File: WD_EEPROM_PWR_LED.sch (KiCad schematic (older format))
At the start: 40 parts, among them IC19 TPS3430WDRCR, IC20 M24C64-DRDW8TP_K, J16 Conn_01x03, Q22 DMN26D0UFB4-7, Q23 DMN26D0UFB4-7, Q24 DMN26D0UFB4-7, Q25 DMN26D0UFB4-7, Q26 DMN26D0UFB4-7, Q27 DMN26D0UFB4-7, Q28 DMN26D0UFB4-7, Q29 DMN26D0UFB4-7

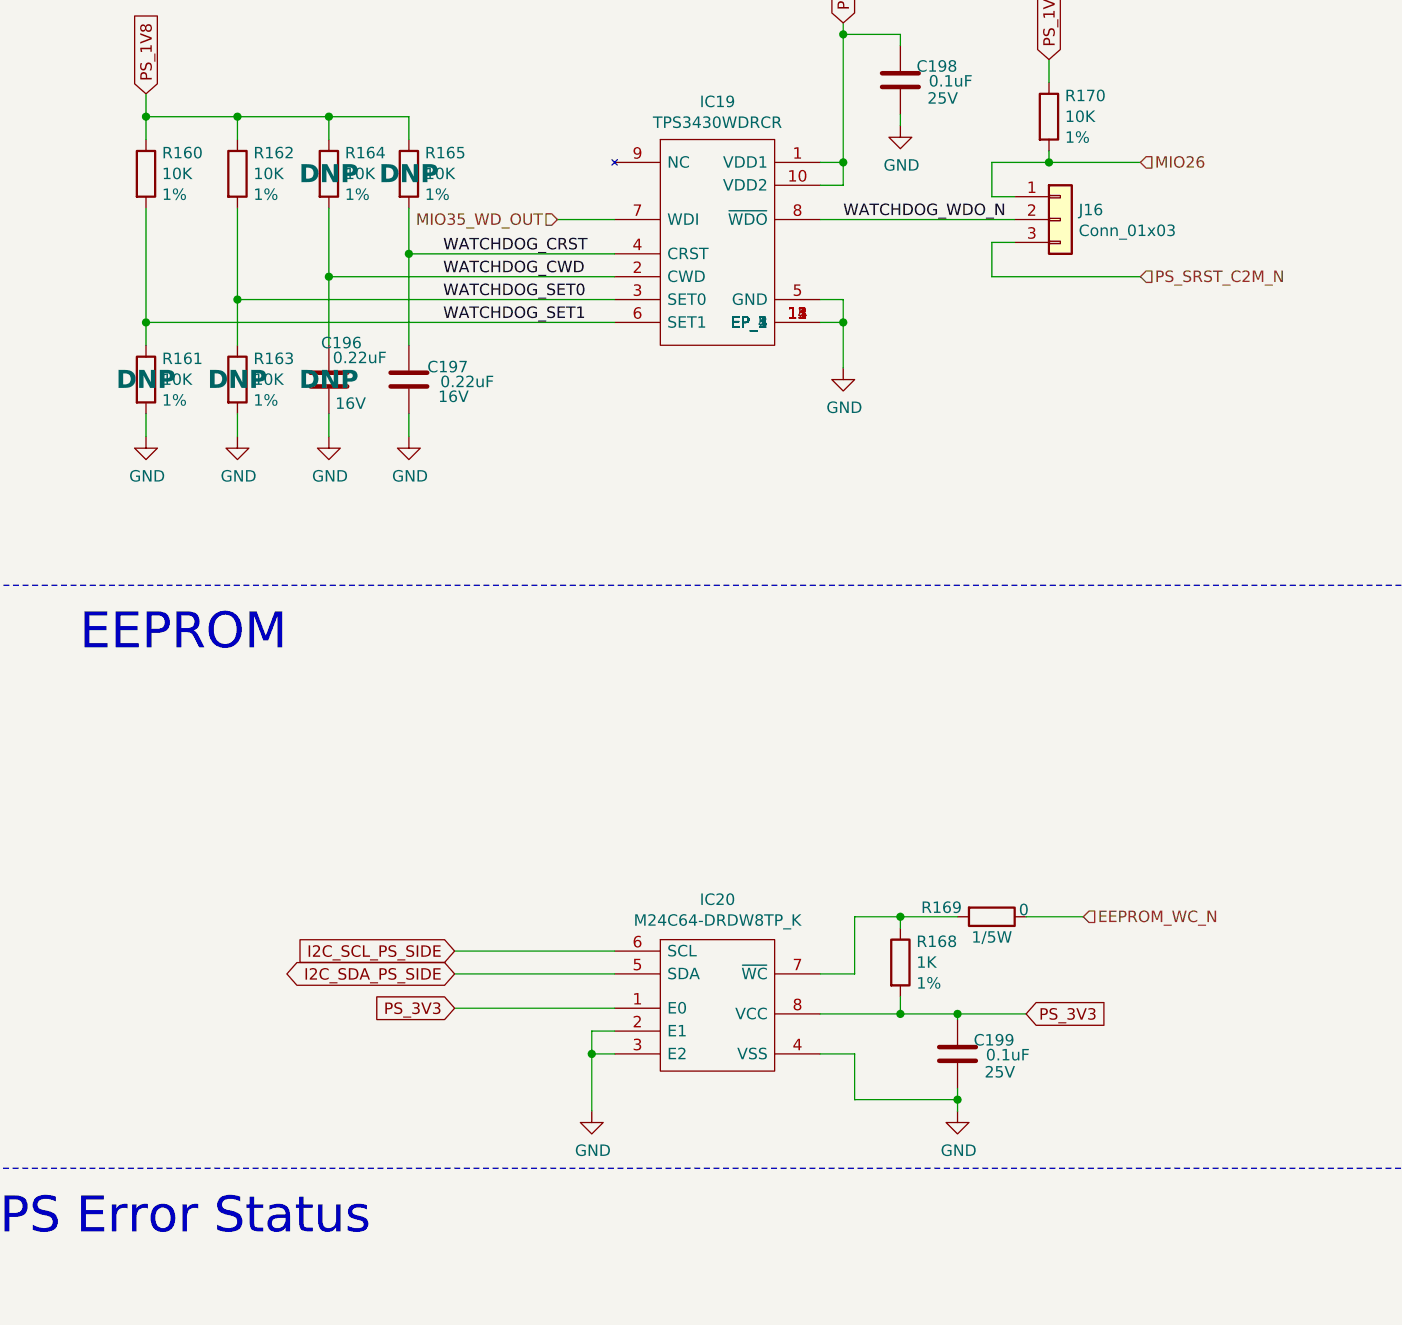
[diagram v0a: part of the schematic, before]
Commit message: Pre-Production Push
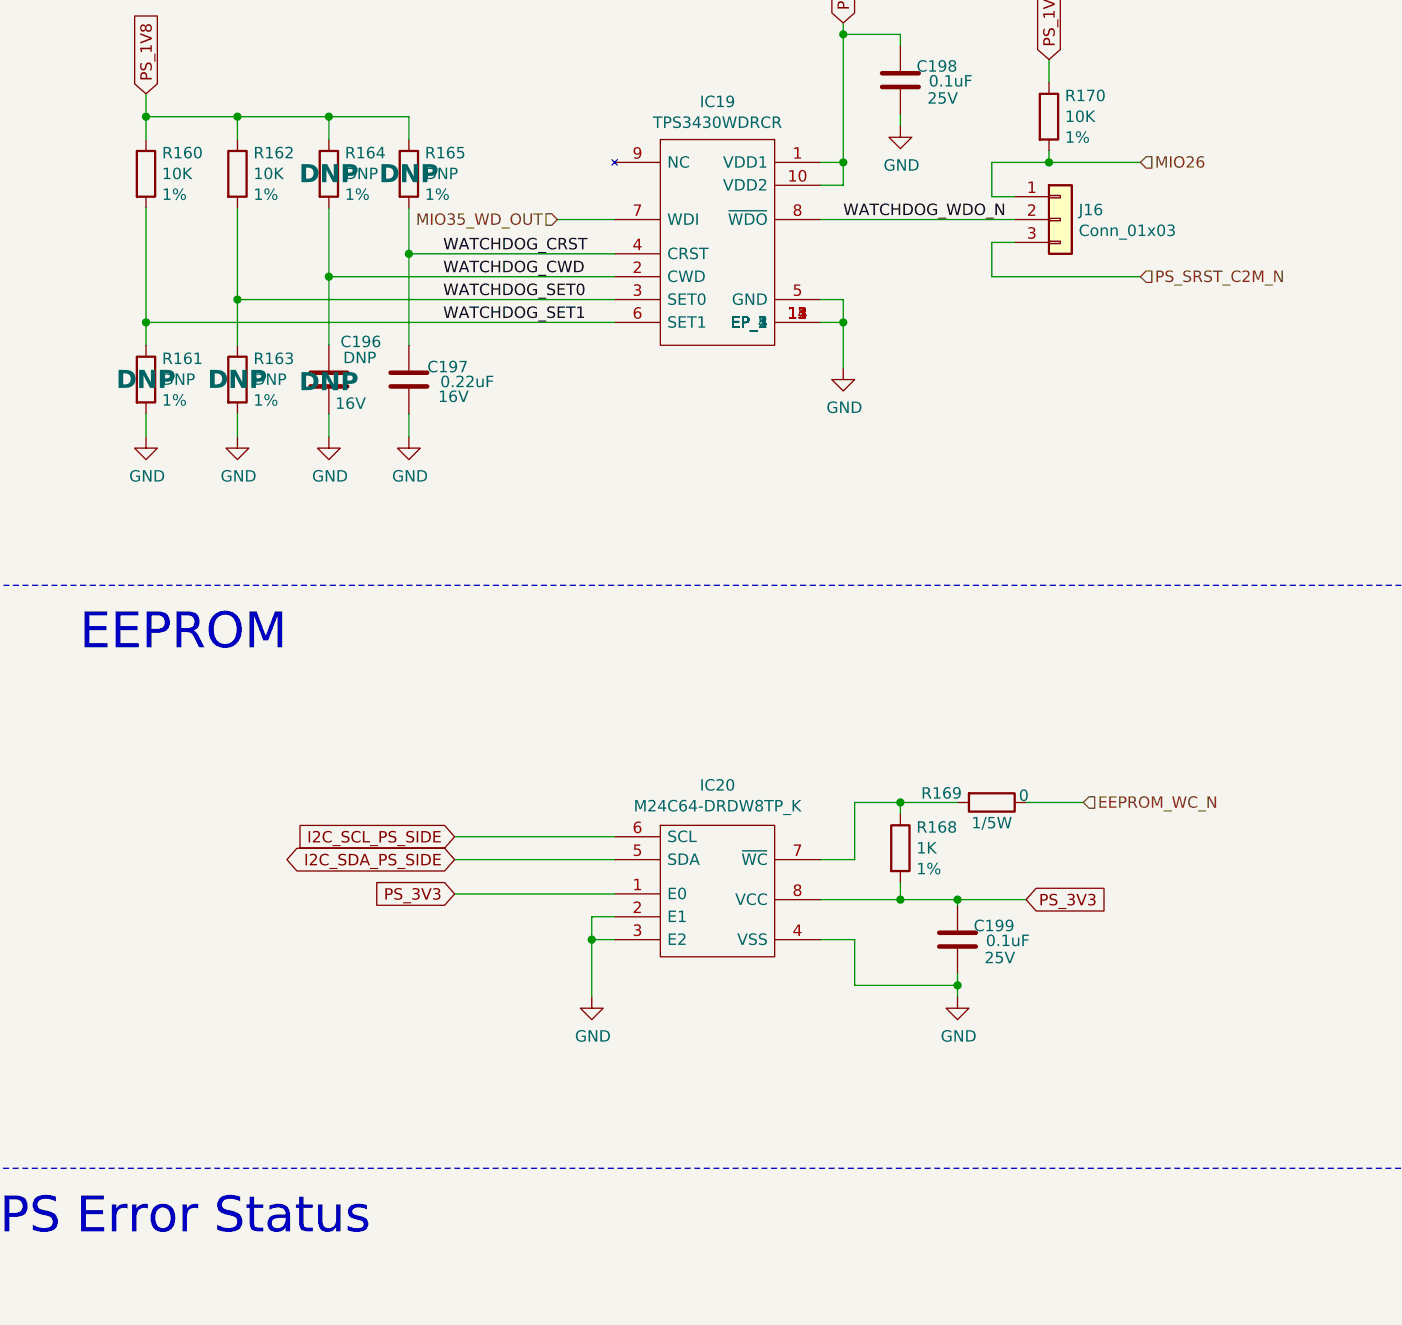
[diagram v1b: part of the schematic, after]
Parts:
- C196: value 0.22uF -> DNP; DNP_Val (none) -> 0.22uF
- R161, R163, R164: value 10K -> DNP
- R165: value 10K -> DNP; DNP_Val (none) -> 10k
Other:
- moved on the sheet: C199, IC20, R168, R169
